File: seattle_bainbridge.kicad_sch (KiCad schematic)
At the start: 12 parts

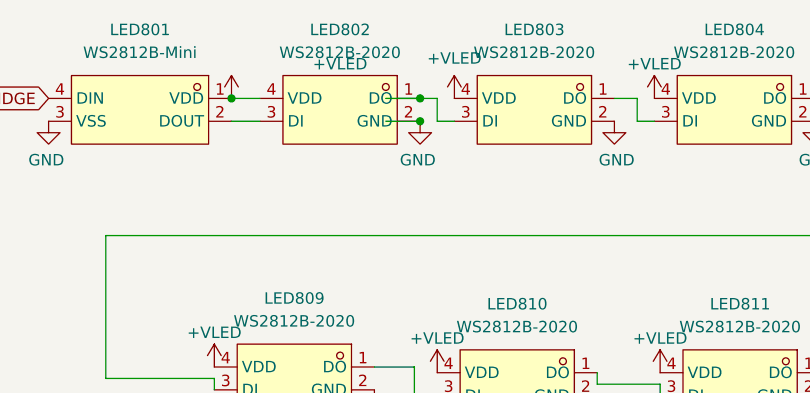
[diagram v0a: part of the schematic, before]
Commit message: rev-b validation run
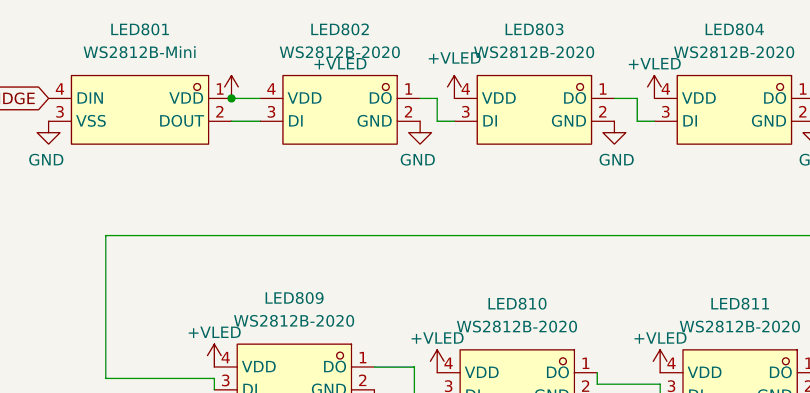
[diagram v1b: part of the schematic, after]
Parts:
- LED802, LED803, LED804, LED805, LED806, LED807, LED808, LED809, LED810, LED811, LED812: LCSC Part C965555 -> C52917434
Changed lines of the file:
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@@
 	(paper "A4")
 	(junction
-		(at 99.695 38.735)
-		(diameter 0)
-		(color 0 0 0 0)
-	)
-	(junction
-		(at 99.695 36.195)
-		(diameter 0)
-		(color 0 0 0 0)
-	)
-	(junction
 		(at 78.74 36.195)
 		(diameter 0)
@@
 	(wire
 		(pts
-			(xy 99.695 38.735) (xy 95.885 38.735)
-		)
-		(stroke
-			(width 0)
-			(type default)
-		)
-	)
-	(wire
-		(pts
 			(xy 146.05 37.465) (xy 146.05 38.735)
 		)
@@
 		)
 	)
-	(wire
-		(pts
-			(xy 95.885 36.195) (xy 99.695 36.195)
-		)
-		(stroke
-			(width 0)
-			(type default)
-		)
-	)
 	(global_label "BAINBRIDGE_X_KINGSTON"
 		(shape input)
@@
 			)
 		)
-		(property "Datasheet" "https://lcsc.com/product-detail/Light-Emitting-Diodes-LED_Worldsemi-WS2812B-2020_C965555.html"
+		(property "Datasheet" "https://lcsc.com/product-detail/Light-Emitting-Diodes-LED_Worldsemi-WS2812B-2020_C52917434.html"
 			(at 119.38 79.375 0)
 			(hide yes)
@@
 			)
 		)
-		(property "LCSC Part" "C965555"
+		(property "LCSC Part" "C52917434"
 			(at 119.38 81.915 0)
 			(hide yes)
@@
 			)
 		)
-		(property "Datasheet" "https://lcsc.com/product-detail/Light-Emitting-Diodes-LED_Worldsemi-WS2812B-2020_C965555.html"
+		(property "Datasheet" "https://lcsc.com/product-detail/Light-Emitting-Diodes-LED_Worldsemi-WS2812B-2020_C52917434.html"
 			(at 168.91 79.375 0)
 			(hide yes)
@@
 			)
 		)
-		(property "LCSC Part" "C965555"
+		(property "LCSC Part" "C52917434"
 			(at 168.91 81.915 0)
 			(hide yes)
@@
 			)
 		)
-		(property "Datasheet" "https://lcsc.com/product-detail/Light-Emitting-Diodes-LED_Worldsemi-WS2812B-2020_C965555.html"
+		(property "Datasheet" "https://lcsc.com/product-detail/Light-Emitting-Diodes-LED_Worldsemi-WS2812B-2020_C52917434.html"
 			(at 143.51 48.895 0)
 			(hide yes)
@@
 			)
 		)
-		(property "LCSC Part" "C965555"
+		(property "LCSC Part" "C52917434"
 			(at 143.51 51.435 0)
 			(hide yes)
@@
 			)
 		)
-		(property "Datasheet" "https://lcsc.com/product-detail/Light-Emitting-Diodes-LED_Worldsemi-WS2812B-2020_C965555.html"
+		(property "Datasheet" "https://lcsc.com/product-detail/Light-Emitting-Diodes-LED_Worldsemi-WS2812B-2020_C52917434.html"
 			(at 144.145 79.375 0)
 			(hide yes)
@@
 			)
 		)
-		(property "LCSC Part" "C965555"
+		(property "LCSC Part" "C52917434"
 			(at 144.145 81.915 0)
 			(hide yes)
@@
 			)
 		)
-		(property "Datasheet" "https://lcsc.com/product-detail/Light-Emitting-Diodes-LED_Worldsemi-WS2812B-2020_C965555.html"
+		(property "Datasheet" "https://lcsc.com/product-detail/Light-Emitting-Diodes-LED_Worldsemi-WS2812B-2020_C52917434.html"
 			(at 99.695 48.895 0)
 			(hide yes)
@@
 			)
 		)
-		(property "LCSC Part" "C965555"
+		(property "LCSC Part" "C52917434"
 			(at 99.695 51.435 0)
 			(hide yes)
@@
 			)
 		)
-		(property "Datasheet" "https://lcsc.com/product-detail/Light-Emitting-Diodes-LED_Worldsemi-WS2812B-2020_C965555.html"
+		(property "Datasheet" "https://lcsc.com/product-detail/Light-Emitting-Diodes-LED_Worldsemi-WS2812B-2020_C52917434.html"
 			(at 186.055 48.895 0)
 			(hide yes)
@@
 			)
 		)
-		(property "LCSC Part" "C965555"
+		(property "LCSC Part" "C52917434"
 			(at 186.055 51.435 0)
 			(hide yes)
@@
 			)
 		)
-		(property "Datasheet" "https://lcsc.com/product-detail/Light-Emitting-Diodes-LED_Worldsemi-WS2812B-2020_C965555.html"
+		(property "Datasheet" "https://lcsc.com/product-detail/Light-Emitting-Diodes-LED_Worldsemi-WS2812B-2020_C52917434.html"
 			(at 231.14 49.53 0)
 			(hide yes)
@@
 			)
 		)
-		(property "LCSC Part" "C965555"
+		(property "LCSC Part" "C52917434"
 			(at 231.14 52.07 0)
 			(hide yes)
@@
 			)
 		)
-		(property "Datasheet" "https://lcsc.com/product-detail/Light-Emitting-Diodes-LED_Worldsemi-WS2812B-2020_C965555.html"
+		(property "Datasheet" "https://lcsc.com/product-detail/Light-Emitting-Diodes-LED_Worldsemi-WS2812B-2020_C52917434.html"
 			(at 121.285 48.895 0)
 			(hide yes)
@@
 			)
 		)
-		(property "LCSC Part" "C965555"
+		(property "LCSC Part" "C52917434"
 			(at 121.285 51.435 0)
 			(hide yes)
@@
 			)
 		)
-		(property "Datasheet" "https://lcsc.com/product-detail/Light-Emitting-Diodes-LED_Worldsemi-WS2812B-2020_C965555.html"
+		(property "Datasheet" "https://lcsc.com/product-detail/Light-Emitting-Diodes-LED_Worldsemi-WS2812B-2020_C52917434.html"
 			(at 163.83 48.895 0)
 			(hide yes)
@@
 			)
 		)
-		(property "LCSC Part" "C965555"
+		(property "LCSC Part" "C52917434"
 			(at 163.83 51.435 0)
 			(hide yes)
@@
 			)
 		)
-		(property "Datasheet" "https://lcsc.com/product-detail/Light-Emitting-Diodes-LED_Worldsemi-WS2812B-2020_C965555.html"
+		(property "Datasheet" "https://lcsc.com/product-detail/Light-Emitting-Diodes-LED_Worldsemi-WS2812B-2020_C52917434.html"
 			(at 94.615 78.74 0)
 			(hide yes)
@@
 			)
 		)
-		(property "LCSC Part" "C965555"
+		(property "LCSC Part" "C52917434"
 			(at 94.615 81.28 0)
 			(hide yes)
@@
 			)
 		)
-		(property "Datasheet" "https://lcsc.com/product-detail/Light-Emitting-Diodes-LED_Worldsemi-WS2812B-2020_C965555.html"
+		(property "Datasheet" "https://lcsc.com/product-detail/Light-Emitting-Diodes-LED_Worldsemi-WS2812B-2020_C52917434.html"
 			(at 208.28 48.895 0)
 			(hide yes)
@@
 			)
 		)
-		(property "LCSC Part" "C965555"
+		(property "LCSC Part" "C52917434"
 			(at 208.28 51.435 0)
 			(hide yes)
